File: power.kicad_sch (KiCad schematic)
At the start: 13 parts, among them J3 Conn_01x02, Q1 CSD17575Q3, U19 LM74502, U7 AMS1117-3.3, U8 AMS1117-5.0

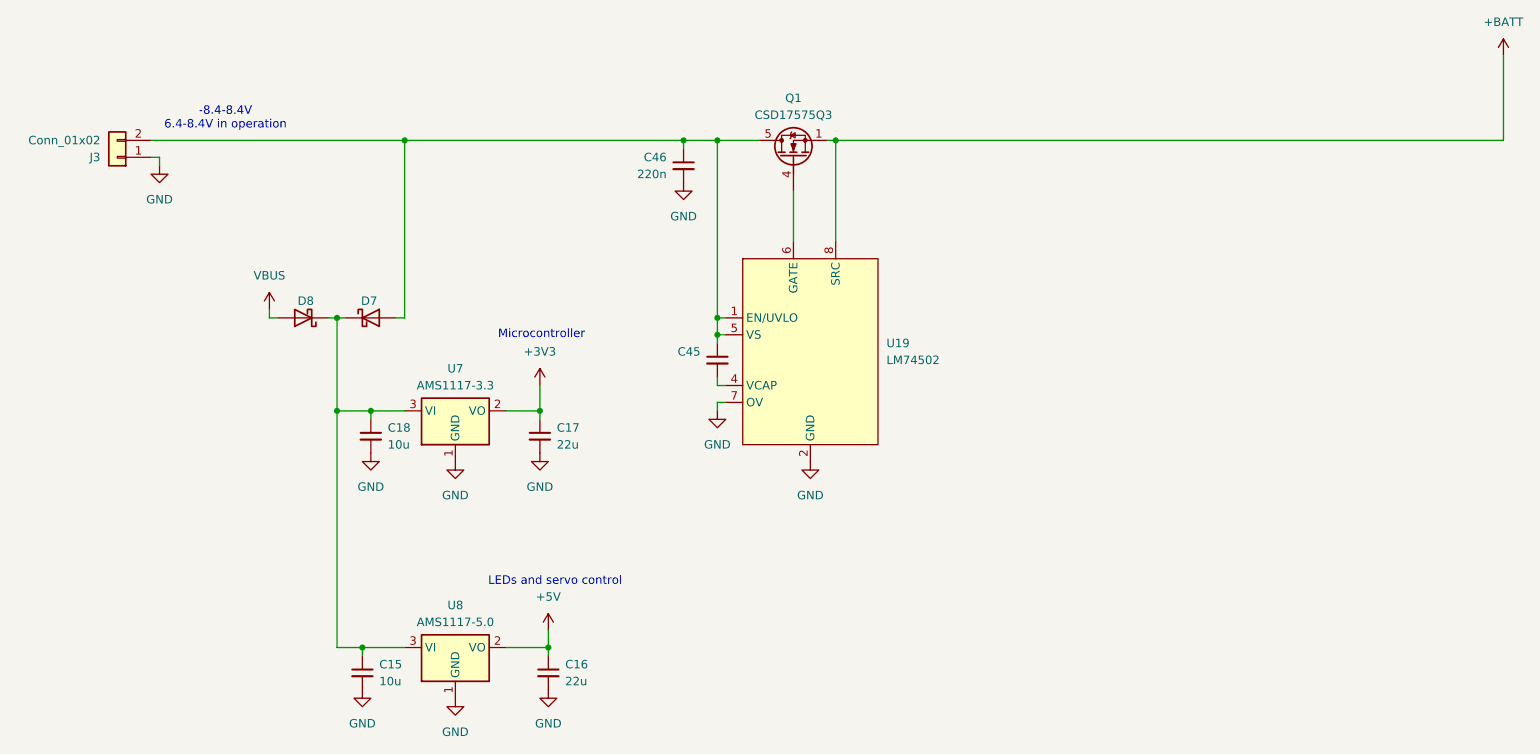
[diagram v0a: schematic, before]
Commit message: changes!
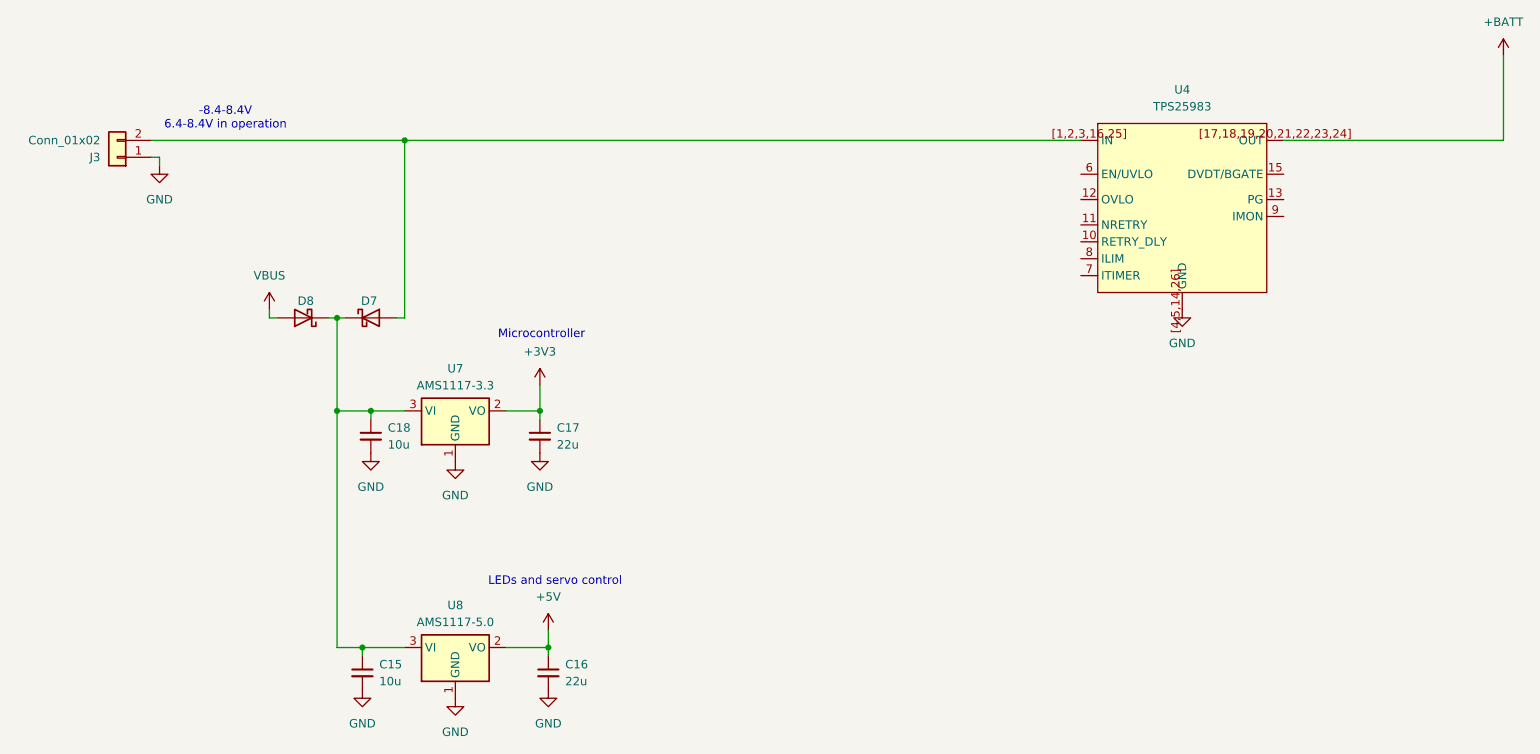
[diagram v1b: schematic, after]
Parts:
- removed C45, C46: 220n, Capacitor_SMD:C_0402_1005Metric, symbol Device:C_Small
- removed Q1: CSD17575Q3, beavs-footprints:SON-8-1EP-3.3x3.3mm-nexfet, symbol Transistor_FET:Q_NMOS_SSSGD_AvalancheRated
- removed U19: LM74502, beavs-footprints:SOT-23-8-THIN, symbol beavs-symbols:LM74502
- added U4: TPS25983, beavs-footprints:Texas_RGE0024M_QFN-24_4x4_Pitch0.5mm_2EP, symbol beavs-symbols:TPS25983
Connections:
- net +BATT: now also U4.[17,18,19,20,21,22,23,24] (OUT)
- net GND: now also U4.[4,5,14,26] (GND)
- net at D7.2 (A), J3.2 (Pin_2): now also U4.[1,2,3,16,25] (IN)
